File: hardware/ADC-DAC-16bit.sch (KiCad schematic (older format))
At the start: 15 parts, among them J1 CON, J2 DAC, J3 ADC, J4 CH1-, J5 CH2-, U1 AD5667R, U2 MCP3426

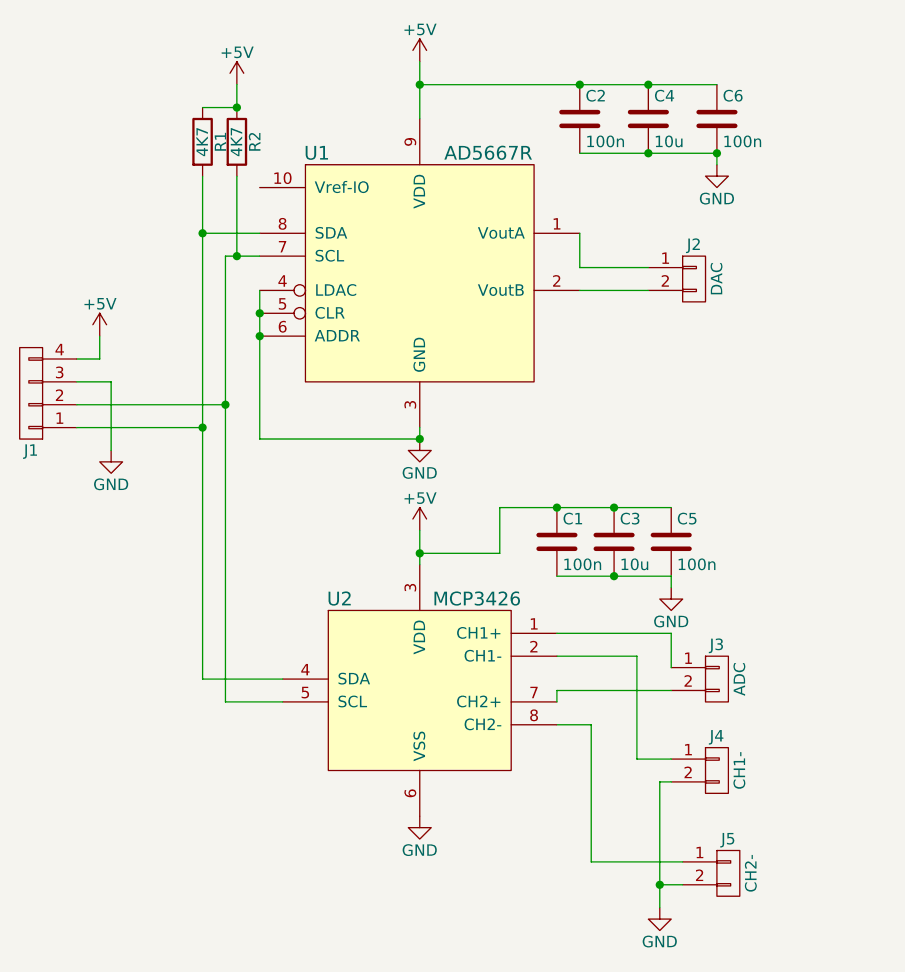
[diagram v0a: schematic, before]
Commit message: v0.2 update
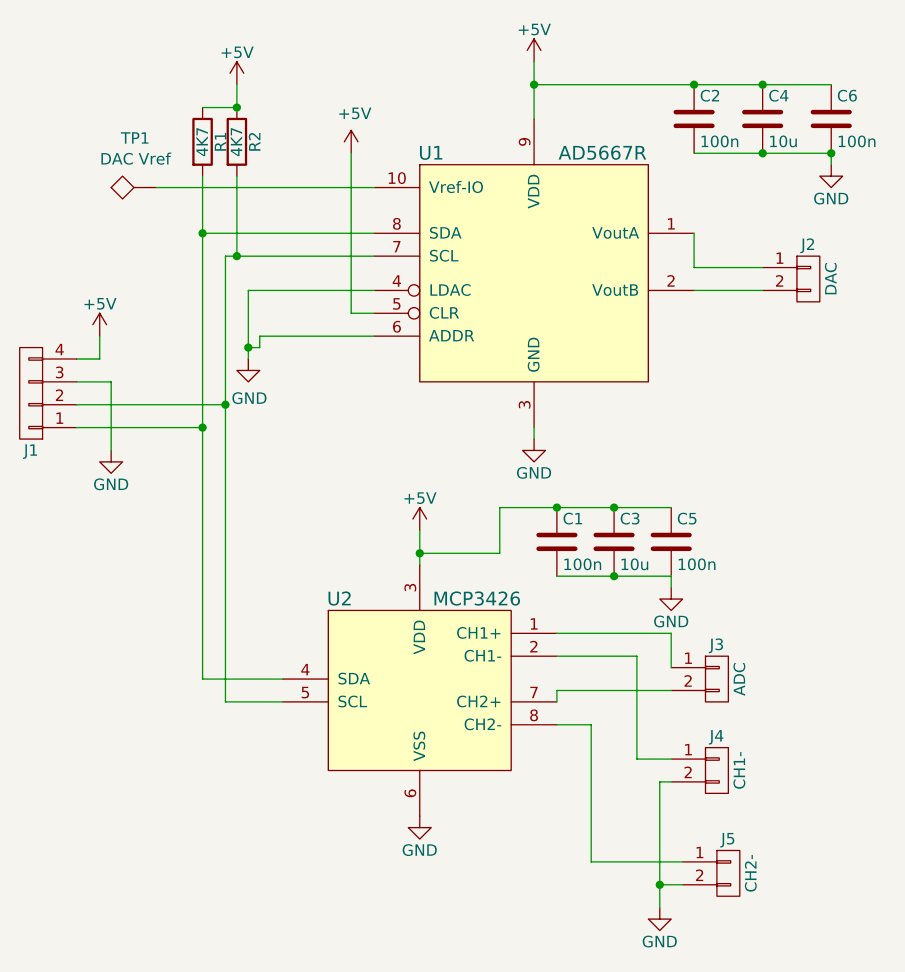
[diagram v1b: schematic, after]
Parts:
- added TP1: DAC Vref, Measurement_Points:Measurement_Point_Round-SMD-Pad_Small, symbol TEST
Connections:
- net +5V: now also U1.5 (CLR)
- net GND: no longer U1.5 (CLR)
- net at U1.10 (Vref-IO): now also TP1.1
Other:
- moved on the sheet: C2, C4, C6, J2, U1
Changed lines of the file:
@@
 LIBS:ADC-DAC-5N44P
 LIBS:ADC-DAC-16bit-cache
-EELAYER 25 0
+EELAYER 26 0
 EELAYER END
 $Descr A4 11693 8268
@@
 L AD5667R U1
 U 1 1 5932A542
-P 2650 2050
-F 0 "U1" H 2200 2800 60  0000 C CNN
-F 1 "AD5667R" H 2950 2800 60  0000 C CNN
-F 2 "Housings_SSOP:MSOP-10_3x3mm_Pitch0.5mm" H 2100 1550 60  0001 C CNN
-F 3 "" H 2100 1550 60  0001 C CNN
-	1    2650 2050
+P 3150 2050
+F 0 "U1" H 2700 2800 60  0000 C CNN
+F 1 "AD5667R" H 3450 2800 60  0000 C CNN
+F 2 "Housings_SSOP:MSOP-10_3x3mm_Pitch0.5mm" H 2600 1550 60  0001 C CNN
+F 3 "" H 2600 1550 60  0001 C CNN
+	1    3150 2050
 	1    0    0    -1
 $EndComp
@@
 $EndComp
 $Comp
-L GND #PWR5
+L GND #PWR01
 U 1 1 5932A544
-P 2650 2550
-F 0 "#PWR5" H 2650 2300 50  0001 C CNN
-F 1 "GND" H 2650 2400 50  0000 C CNN
-F 2 "" H 2650 2550 50  0001 C CNN
-F 3 "" H 2650 2550 50  0001 C CNN
-	1    2650 2550
-	1    0    0    -1
-$EndComp
-$Comp
-L GND #PWR7
+P 3150 2550
+F 0 "#PWR01" H 3150 2300 50  0001 C CNN
+F 1 "GND" H 3150 2400 50  0000 C CNN
+F 2 "" H 3150 2550 50  0001 C CNN
+F 3 "" H 3150 2550 50  0001 C CNN
+	1    3150 2550
+	1    0    0    -1
+$EndComp
+$Comp
+L GND #PWR02
 U 1 1 5932A545
 P 2650 4200
-F 0 "#PWR7" H 2650 3950 50  0001 C CNN
+F 0 "#PWR02" H 2650 3950 50  0001 C CNN
 F 1 "GND" H 2650 4050 50  0000 C CNN
 F 2 "" H 2650 4200 50  0001 C CNN
@@
 $EndComp
 Wire Wire Line
-	1950 1650 1700 1650
+	2450 1650 1700 1650
 Wire Wire Line
 	1700 1400 1700 3600
@@
 	1800 1750 1800 3700
 Wire Wire Line
-	1800 1750 1950 1750
-Wire Wire Line
-	1950 1900 1950 2550
-Connection ~ 1950 2000
-Wire Wire Line
-	2650 2550 2650 2500
-Wire Wire Line
-	1950 2550 2650 2550
-Connection ~ 1950 2100
-Connection ~ 2650 2550
-$Comp
-L +5V #PWR6
+	1800 1750 2450 1750
+Wire Wire Line
+	3150 2550 3150 2500
+$Comp
+L +5V #PWR03
 U 1 1 5932A546
 P 2650 2950
-F 0 "#PWR6" H 2650 2800 50  0001 C CNN
+F 0 "#PWR03" H 2650 2800 50  0001 C CNN
 F 1 "+5V" H 2650 3090 50  0000 C CNN
 F 2 "" H 2650 2950 50  0001 C CNN
@@
 $EndComp
 $Comp
-L +5V #PWR4
+L +5V #PWR04
 U 1 1 5932A547
-P 2650 900
-F 0 "#PWR4" H 2650 750 50  0001 C CNN
-F 1 "+5V" H 2650 1040 50  0000 C CNN
-F 2 "" H 2650 900 50  0001 C CNN
-F 3 "" H 2650 900 50  0001 C CNN
-	1    2650 900
+P 3150 900
+F 0 "#PWR04" H 3150 750 50  0001 C CNN
+F 1 "+5V" H 3150 1040 50  0000 C CNN
+F 2 "" H 3150 900 50  0001 C CNN
+F 3 "" H 3150 900 50  0001 C CNN
+	1    3150 900
 	1    0    0    -1
 $EndComp
@@
 	1700 1100 1850 1100
 $Comp
-L +5V #PWR3
+L +5V #PWR05
 U 1 1 5932A54A
 P 1850 1000
-F 0 "#PWR3" H 1850 850 50  0001 C CNN
+F 0 "#PWR05" H 1850 850 50  0001 C CNN
 F 1 "+5V" H 1850 1140 50  0000 C CNN
 F 2 "" H 1850 1000 50  0001 C CNN
@@
 	1300 2300 1300 2600
 $Comp
-L GND #PWR2
+L GND #PWR06
 U 1 1 5932A54C
 P 1300 2600
-F 0 "#PWR2" H 1300 2350 50  0001 C CNN
+F 0 "#PWR06" H 1300 2350 50  0001 C CNN
 F 1 "GND" H 1300 2450 50  0000 C CNN
 F 2 "" H 1300 2600 50  0001 C CNN
@@
 $EndComp
 $Comp
-L +5V #PWR1
+L +5V #PWR07
 U 1 1 5932A54D
 P 1250 2100
-F 0 "#PWR1" H 1250 1950 50  0001 C CNN
+F 0 "#PWR07" H 1250 1950 50  0001 C CNN
 F 1 "+5V" H 1250 2240 50  0000 C CNN
 F 2 "" H 1250 2100 50  0001 C CNN
@@
 	1250 2200 1250 2100
 $Comp
-L GND #PWR8
+L GND #PWR08
 U 1 1 5932A54E
 P 3700 4600
-F 0 "#PWR8" H 3700 4350 50  0001 C CNN
+F 0 "#PWR08" H 3700 4350 50  0001 C CNN
 F 1 "GND" H 3700 4450 50  0000 C CNN
 F 2 "" H 3700 4600 50  0001 C CNN
@@
 L CONN_01X02 J2
 U 1 1 5932A550
-P 3850 1850
-F 0 "J2" H 3850 2000 50  0000 C CNN
-F 1 "DAC" V 3950 1850 50  0000 C CNN
-F 2 "Pin_Headers:Pin_Header_Straight_1x02_Pitch2.54mm" H 3850 1850 50  0001 C CNN
-F 3 "" H 3850 1850 50  0001 C CNN
-	1    3850 1850
-	1    0    0    -1
-$EndComp
-Wire Wire Line
-	3350 1900 3650 1900
-Wire Wire Line
-	3650 1800 3350 1800
-Wire Wire Line
-	3350 1800 3350 1650
+P 4350 1850
+F 0 "J2" H 4350 2000 50  0000 C CNN
+F 1 "DAC" V 4450 1850 50  0000 C CNN
+F 2 "Pin_Headers:Pin_Header_Straight_1x02_Pitch2.54mm" H 4350 1850 50  0001 C CNN
+F 3 "" H 4350 1850 50  0001 C CNN
+	1    4350 1850
+	1    0    0    -1
+$EndComp
+Wire Wire Line
+	3850 1900 4150 1900
+Wire Wire Line
+	4150 1800 3850 1800
+Wire Wire Line
+	3850 1800 3850 1650
 Wire Wire Line
 	3250 3400 3750 3400
@@
 L C C2
 U 1 1 5932A551
-P 3350 1150
-F 0 "C2" H 3375 1250 50  0000 L CNN
-F 1 "100n" H 3375 1050 50  0000 L CNN
-F 2 "Capacitors_SMD:C_0805_HandSoldering" H 3388 1000 50  0001 C CNN
-F 3 "" H 3350 1150 50  0001 C CNN
-	1    3350 1150
+P 3850 1150
+F 0 "C2" H 3875 1250 50  0000 L CNN
+F 1 "100n" H 3875 1050 50  0000 L CNN
+F 2 "Capacitors_SMD:C_0805_HandSoldering" H 3888 1000 50  0001 C CNN
+F 3 "" H 3850 1150 50  0001 C CNN
+	1    3850 1150
 	1    0    0    -1
 $EndComp
@@
 L C C4
 U 1 1 5932A552
-P 3650 1150
-F 0 "C4" H 3675 1250 50  0000 L CNN
-F 1 "10u" H 3675 1050 50  0000 L CNN
-F 2 "Capacitors_SMD:C_1206_HandSoldering" H 3688 1000 50  0001 C CNN
-F 3 "" H 3650 1150 50  0001 C CNN
-	1    3650 1150
+P 4150 1150
+F 0 "C4" H 4175 1250 50  0000 L CNN
+F 1 "10u" H 4175 1050 50  0000 L CNN
+F 2 "Capacitors_SMD:C_1206_HandSoldering" H 4188 1000 50  0001 C CNN
+F 3 "" H 4150 1150 50  0001 C CNN
+	1    4150 1150
 	1    0    0    -1
 $EndComp
@@
 L C C6
 U 1 1 5932A553
-P 3950 1150
-F 0 "C6" H 3975 1250 50  0000 L CNN
-F 1 "100n" H 3975 1050 50  0000 L CNN
-F 2 "Capacitors_SMD:C_0603_HandSoldering" H 3988 1000 50  0001 C CNN
-F 3 "" H 3950 1150 50  0001 C CNN
-	1    3950 1150
+P 4450 1150
+F 0 "C6" H 4475 1250 50  0000 L CNN
+F 1 "100n" H 4475 1050 50  0000 L CNN
+F 2 "Capacitors_SMD:C_0603_HandSoldering" H 4488 1000 50  0001 C CNN
+F 3 "" H 4450 1150 50  0001 C CNN
+	1    4450 1150
 	1    0    0    -1
 $EndComp
@@
 	3750 3150 3750 3200
 $Comp
-L GND #PWR9
+L GND #PWR09
 U 1 1 5932A557
 P 3750 3200
-F 0 "#PWR9" H 3750 2950 50  0001 C CNN
+F 0 "#PWR09" H 3750 2950 50  0001 C CNN
 F 1 "GND" H 3750 3050 50  0000 C CNN
 F 2 "" H 3750 3200 50  0001 C CNN
@@
 $EndComp
 Wire Wire Line
-	2650 1000 3950 1000
-Connection ~ 3650 1000
-Wire Wire Line
-	2650 900  2650 1150
-Connection ~ 3350 1000
-Connection ~ 2650 1000
-Wire Wire Line
-	3350 1300 3950 1300
-Connection ~ 3650 1300
-$Comp
-L GND #PWR10
+	3150 1000 4450 1000
+Connection ~ 4150 1000
+Wire Wire Line
+	3150 900  3150 1150
+Connection ~ 3850 1000
+Connection ~ 3150 1000
+Wire Wire Line
+	3850 1300 4450 1300
+Connection ~ 4150 1300
+$Comp
+L GND #PWR010
 U 1 1 5932A558
-P 3950 1350
-F 0 "#PWR10" H 3950 1100 50  0001 C CNN
-F 1 "GND" H 3950 1200 50  0000 C CNN
-F 2 "" H 3950 1350 50  0001 C CNN
-F 3 "" H 3950 1350 50  0001 C CNN
-	1    3950 1350
-	1    0    0    -1
-$EndComp
-Wire Wire Line
-	3950 1300 3950 1350
-Connection ~ 3950 1300
+P 4450 1350
+F 0 "#PWR010" H 4450 1100 50  0001 C CNN
+F 1 "GND" H 4450 1200 50  0000 C CNN
+F 2 "" H 4450 1350 50  0001 C CNN
+F 3 "" H 4450 1350 50  0001 C CNN
+	1    4450 1350
+	1    0    0    -1
+$EndComp
+Wire Wire Line
+	4450 1300 4450 1350
+Connection ~ 4450 1300
 $Comp
 L CONN_01X02 J4
@@
 Wire Wire Line
 	3600 3500 3250 3500
+Wire Wire Line
+	2450 2000 2350 2000
+Wire Wire Line
+	2350 2000 2350 1300
+$Comp
+L +5V #PWR011
+U 1 1 596D2637
+P 2350 1300
+F 0 "#PWR011" H 2350 1150 50  0001 C CNN
+F 1 "+5V" H 2365 1473 50  0000 C CNN
+F 2 "" H 2350 1300 50  0001 C CNN
+F 3 "" H 2350 1300 50  0001 C CNN
+	1    2350 1300
+	1    0    0    -1
+$EndComp
+Wire Wire Line
+	2450 1450 1500 1450
+$Comp
+L TEST TP1
+U 1 1 596D2C65
+P 1500 1450
+F 0 "TP1" V 1715 1544 50  0000 C CNN
+F 1 "DAC Vref" V 1624 1544 50  0000 C CNN
+F 2 "Measurement_Points:Measurement_Point_Round-SMD-Pad_Small" H 1500 1450 50  0001 C CNN
+F 3 "" H 1500 1450 50  0001 C CNN
+	1    1500 1450
+	0    -1   -1   0
+$EndComp
+Wire Wire Line
+	1900 1900 1900 2200
+Wire Wire Line
+	1950 2100 2450 2100
+Wire Wire Line
+	1950 2100 1950 2150
+Wire Wire Line
+	1950 2150 1900 2150
+Connection ~ 1900 2150
+$Comp
+L GND #PWR012
+U 1 1 596D5752
+P 1900 2200
+F 0 "#PWR012" H 1900 1950 50  0001 C CNN
+F 1 "GND" H 1905 2027 50  0000 C CNN
+F 2 "" H 1900 2200 50  0001 C CNN
+F 3 "" H 1900 2200 50  0001 C CNN
+	1    1900 2200
+	1    0    0    -1
+$EndComp
+Wire Wire Line
+	2450 1900 1900 1900
 $EndSCHEMATC
